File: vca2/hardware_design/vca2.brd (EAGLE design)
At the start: 29.2 x 100 mm, 112 parts, among them IC1 LM13700M, IC2 NCS20074D, IC3 TL074D, IC4 TL072D, IC5 NCS20074D, T1 2N3906, T2 BC847BS, T3 2N3906, T4 2N3906, T5 BC847BS, T6 2N3906

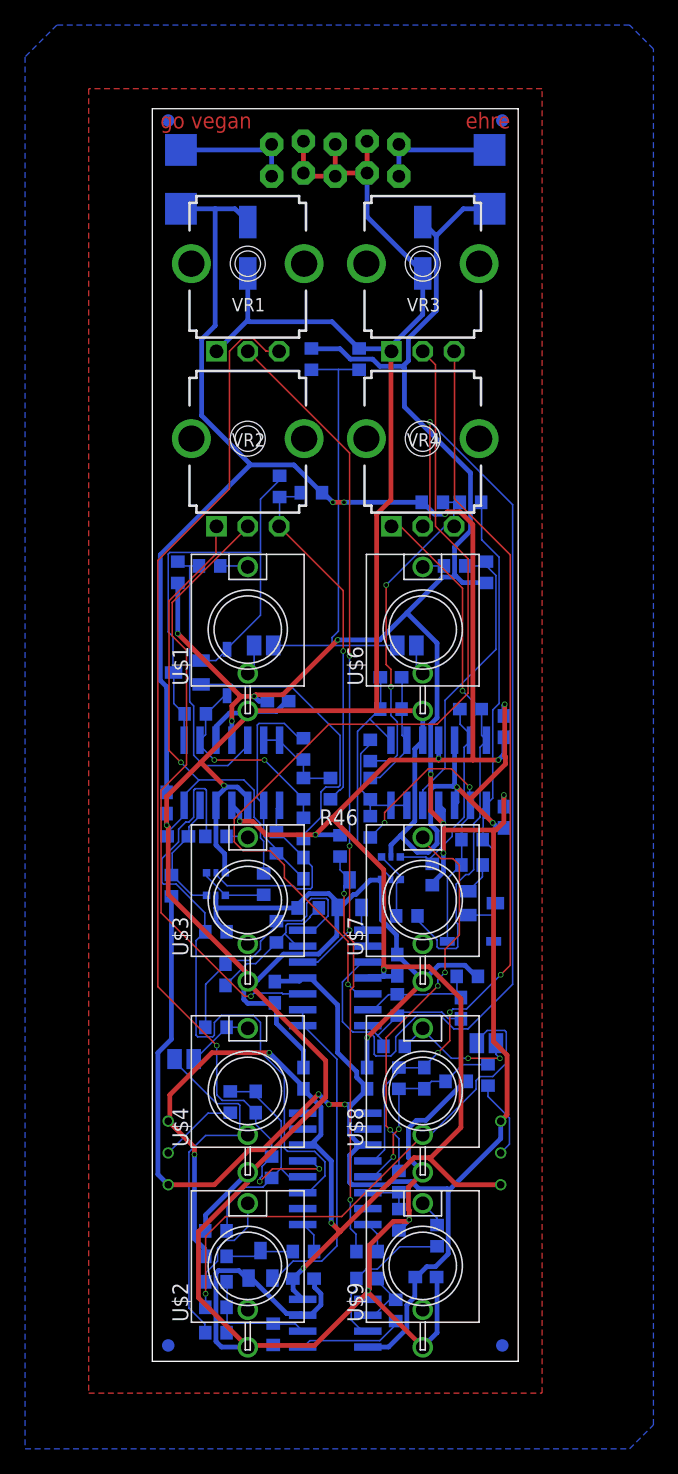
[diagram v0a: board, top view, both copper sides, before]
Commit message: New version of vca2 with manufacturing parts. This is the first dirty version!!!!!
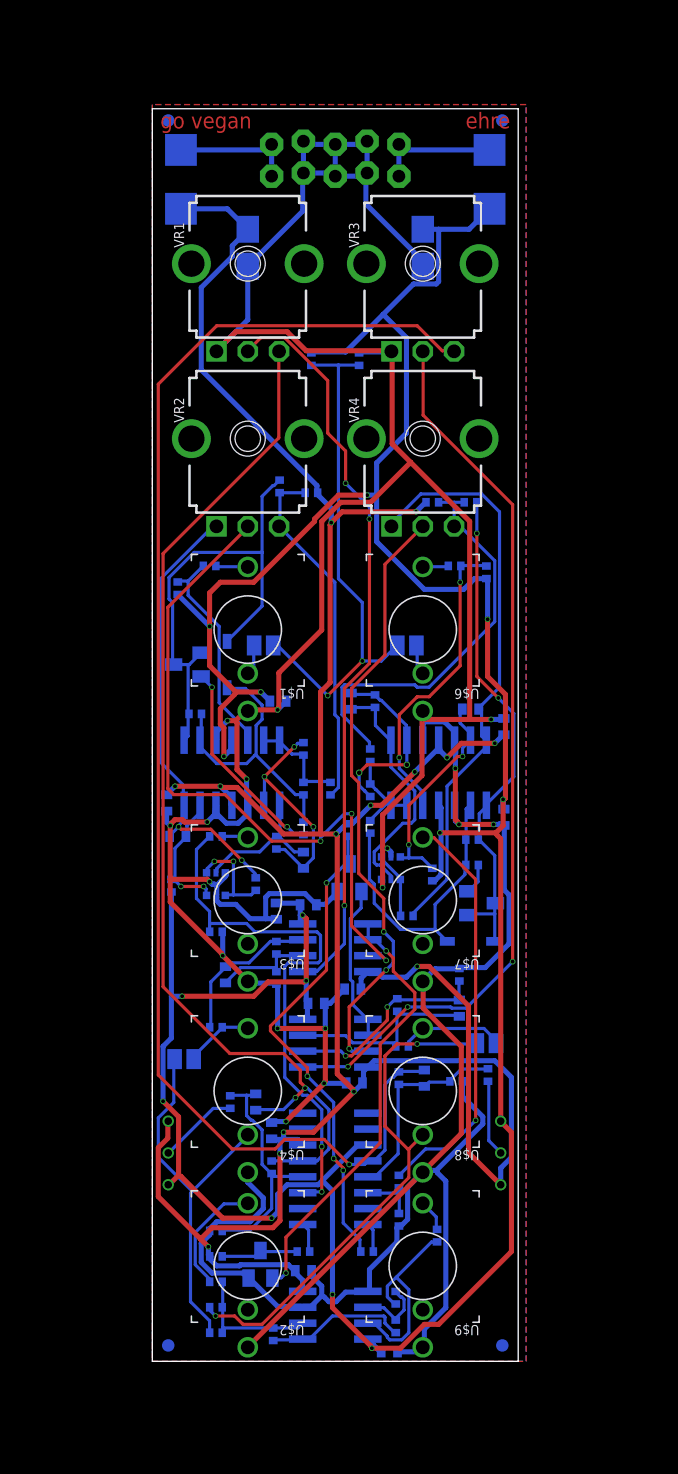
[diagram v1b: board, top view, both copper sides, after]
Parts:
- removed C6, C7: 22uF, rcl:PANASONIC_C
- removed IC3: TL074D, linear:SO14
- added C22, C23: 100nF, jhbruhn-cr:C0402
- added C24, C25: 10uF, rcl:A/3216-18W
- added U1, U2: TL072CD, jhbruhn-opamp:SOIC8
- C1: device MusicThingModular:EURO_PWR_HEADER_LOCK -> jhbruhn-physical:EURO_PWR_HEADER_LOCK
- C10, C11, C12, C13, C14, C15, C16, C17, C18, C19, C2, C20, C21, C3, C4, C5, C8, C9: device rcl:C0603 -> jhbruhn-cr:C0402
- IC1: device ota:SO16 -> jhbruhn-ota:SO16
- IC4: value TL072D -> TL072CD; device linear:SO08 -> jhbruhn-opamp:SOIC8
- R1, R10, R11, R12, R13, R15, R16, R17, R19, R2, R20, R21, R22, R23, R24, R25, R26, R27, R28, R29, R3, R30, R31, R32, R33, R34, R35, R36, R38, R39, R4, R40, R42, R43, R44, R45, R46, R47, R48, R49, R5, R50, R51, R52, R53, R54, R55, R6, R7, R8, R9: device rcl:R0603 -> jhbruhn-cr:R0402
- R14, R37: value 600R -> 680R; device rcl:R0603 -> jhbruhn-cr:R0402
- U$1, U$2, U$3, U$4, U$6, U$7, U$8, U$9: device thonkiconn:WQP-PJ301M-12_JACK -> jhbruhn-physical:WQP-PJ301M-12_JACK
- VR1, VR2, VR3, VR4: device MusicThingModular:9MM_SNAP-IN_POT -> jhbruhn-physical:9MM_SNAP-IN_POT
- moved C2 7.22 mm to (13.1, 28.6), turned to 180 degrees
- moved C20 6.65 mm to (18.9, 0.76)
- moved C16 6.48 mm to (9.91, 35.9)
- moved R20 6.14 mm to (9.91, 30.6), turned to 270 degrees
- moved C3 4.08 mm to (16.1, 22.2), turned to 180 degrees
- moved C17 4.03 mm to (16.0, 29.7), turned to 180 degrees
- moved C12 3.70 mm to (15.9, 52.7), turned to 90 degrees
- moved R48 2.75 mm to (19.4, 5.08), turned to 270 degrees
- moved R33 1.42 mm to (17.8, 52.7), turned to 270 degrees
- moved R46 1.42 mm to (15.6, 42.4)
- moved R49 1.27 mm to (19.4, 2.79)
- moved R19 1.27 mm to (9.91, 33.0)
- moved R2 1.27 mm to (2.03, 61.7)
- moved T6 1.27 mm to (15.7, 38.6)
- moved R43 0.65 mm to (24.5, 30.9), turned to 90 degrees
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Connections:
- net +12V: now also C22.1, C24.+, U1.8, U2.8; no longer C6.+, IC3.4
- net -12V: now also C23.2, C25.-, U1.4, U2.4; no longer C7.-, IC3.11
- net CHANNEL_A: now also U$4.P$1_TIP; no longer U$4.P$1
- net CHANNEL_A_OUT: now also U$4.P$2_SWITCH; no longer U$4.P$2
- net CHANNEL_B: now also U$8.P$1_TIP; no longer U$8.P$1
- net CHANNEL_B_OUT: now also U$8.P$2_SWITCH; no longer U$8.P$2
- net GND: now also C22.2, C23.1, C24.-, C25.+, U$1.P$3_SLEEVE, U$2.P$3_SLEEVE, U$3.P$3_SLEEVE, U$4.P$3_SLEEVE, U$6.P$3_SLEEVE, U$7.P$3_SLEEVE, U$8.P$3_SLEEVE, U$9.P$3_SLEEVE; no longer C6.-, C7.+, U$1.P$3, U$2.P$3, U$3.P$3, U$4.P$3, U$6.P$3, U$7.P$3, U$8.P$3, U$9.P$3
- net N$14: now also U$3.P$1_TIP; no longer U$3.P$1
- net N$16: now also U$9.P$1_TIP; no longer U$9.P$1
- net N$19: now also U1.5; no longer IC3.5
- net N$20: now also U1.6; no longer IC3.6
- net N$22: now also U1.7; no longer IC3.7
- net N$23: now also U1.1, U1.2; no longer IC3.1, IC3.2
- net N$24: now also U1.3; no longer IC3.3
- net N$29: now also U$6.P$1_TIP; no longer U$6.P$1
- net N$38: now also U$7.P$1_TIP; no longer U$7.P$1
- net N$4: now also U$1.P$1_TIP; no longer U$1.P$1
- net N$45: now also U2.6; no longer IC3.13
- net N$46: now also U2.5; no longer IC3.12
- net N$47: now also U2.7; no longer IC3.14
- net N$49: now also U2.1, U2.2; no longer IC3.8, IC3.9
- net N$50: now also U2.3; no longer IC3.10
- net N$56: now also U$1.P$2_SWITCH; no longer U$1.P$2
- net N$57: now also U$2.P$1_TIP; no longer U$2.P$1
- net N$58: now also U$6.P$2_SWITCH; no longer U$6.P$2
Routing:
- net N$43: track 73.3 -> 112.6 mm, vias 3 -> 1
- net N$50: track 81.5 -> 48.5 mm, vias 1 -> 3
- net +12V: track 240.7 -> 259.0 mm, vias 11 -> 14
- net GND: track 361.2 -> 374.3 mm, vias 8 -> 17
- net N$49: track 3.34 -> 12.4 mm
- net N$23: track 26.2 -> 35.3 mm, vias 0 -> 2
- net N$15: track 52.7 -> 43.8 mm, vias 0 -> 2
- net N$22: track 21.1 -> 12.5 mm
- net -12V: track 230.6 -> 222.1 mm, vias 12 -> 14
- net N$45: track 9.94 -> 16.7 mm, vias 0 -> 2
- net N$24: track 48.9 -> 55.5 mm, vias 1 -> 3
- net N$30: track 27.0 -> 33.6 mm, vias 2 -> 0
- net N$52: track 32.7 -> 39.1 mm, vias 2 -> 4
- net N$8: track 22.9 -> 16.5 mm, vias 0 -> 2
- net N$11: track 16.6 -> 22.9 mm, vias 2 -> 0
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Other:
- board text added: "jhbruhn 2020"
- board text removed: "jhbruhn 2019"
